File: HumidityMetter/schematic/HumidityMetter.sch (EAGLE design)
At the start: 65 parts, among them IC1 LM317, IC2 LM317, IC3 STM32F103C8T6, IC4 AM2320, J1 0, J2 0, J3 0, J4 0, K1 POWER_ON, T1 BSS84, T2 BC847, X1 +9V, X2 GND, X3 ISP

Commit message: Himidity metter. Board routed.
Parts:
- R24: device __MyCommonLib1:RSMD_0805 -> __MyCommonLib1:RSMD_1206_BIG_GAP
- R26, R27, R28, R29: device __MyCommonLib1:RSMD_0805 -> __MyCommonLib1:R0207
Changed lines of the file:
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@@
 <setting verticaltext="up"/>
 </settings>
-<grid distance="0.025" unitdist="inch" unit="inch" style="lines" multiple="4" display="yes" altdistance="0.01" altunitdist="inch" altunit="inch"/>
+<grid distance="0.1" unitdist="inch" unit="inch" style="lines" multiple="1" display="no" altdistance="0.01" altunitdist="inch" altunit="inch"/>
 <layers>
 <layer number="1" name="Top" color="4" fill="1" visible="yes" active="no"/>
@@
 <part name="R22" library="__MyCommonLib1" deviceset="R" device="SMD_0805" value="390R"/>
 <part name="R23" library="__MyCommonLib1" deviceset="R" device="SMD_0805" value="390R"/>
-<part name="R24" library="__MyCommonLib1" deviceset="R" device="SMD_0805" value="18K"/>
+<part name="R24" library="__MyCommonLib1" deviceset="R" device="SMD_1206_BIG_GAP" value="18K"/>
 <part name="R25" library="__MyCommonLib1" deviceset="R" device="SMD_0805" value="6K8"/>
 <part name="C9" library="__MyCommonLib1" deviceset="C" device="SMD_0805" value="0.1uF"/>
@@
 <part name="C1" library="__MyCommonLib1" deviceset="C" device="SMD_0805" value="0.1uF"/>
 <part name="GND28" library="supply1" deviceset="GND" device=""/>
-<part name="R26" library="__MyCommonLib1" deviceset="R" device="SMD_0805" value="4K7"/>
-<part name="R27" library="__MyCommonLib1" deviceset="R" device="SMD_0805" value="4K7"/>
-<part name="R28" library="__MyCommonLib1" deviceset="R" device="SMD_0805" value="200R"/>
-<part name="R29" library="__MyCommonLib1" deviceset="R" device="SMD_0805" value="200R"/>
+<part name="R26" library="__MyCommonLib1" deviceset="R" device="0207" value="4K7"/>
+<part name="R27" library="__MyCommonLib1" deviceset="R" device="0207" value="4K7"/>
+<part name="R28" library="__MyCommonLib1" deviceset="R" device="0207" value="200R"/>
+<part name="R29" library="__MyCommonLib1" deviceset="R" device="0207" value="200R"/>
 <part name="D10" library="__MyCommonLib1" deviceset="1N4001" device="DO-41_10MM" value="1N4007"/>
 <part name="GND29" library="supply1" deviceset="GND" device=""/>

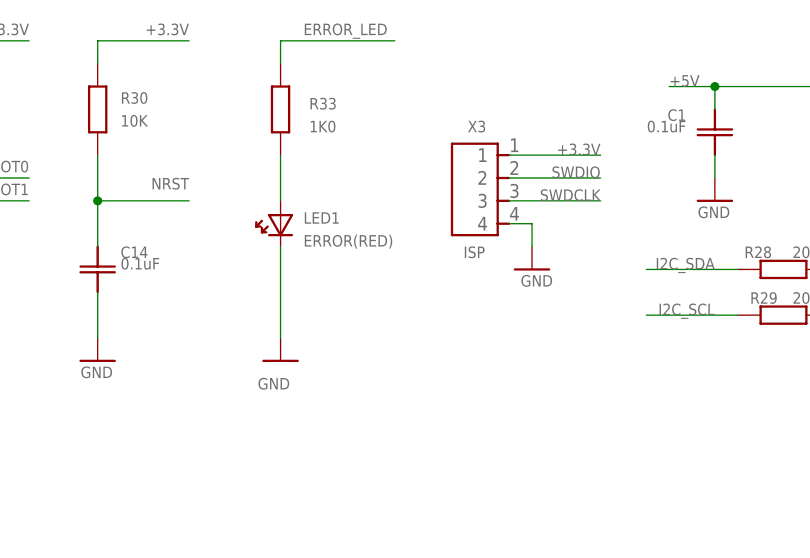
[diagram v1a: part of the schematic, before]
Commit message: Himidity metter. Board routed.
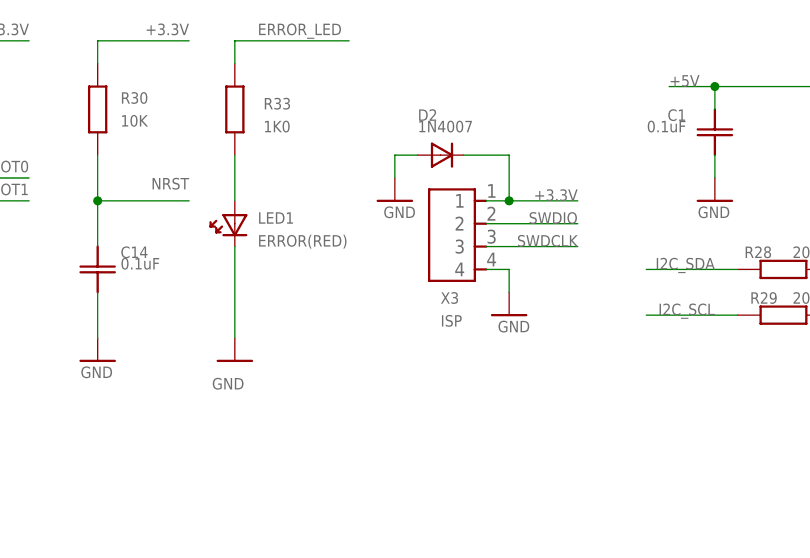
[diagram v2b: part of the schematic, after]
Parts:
- added D2: 1N4007, __MyCommonLib1:1N4001DO-41_10MM
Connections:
- net +3.3V: now also D2.CATHODE
- net GND: now also D2.ANODE
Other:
- moved on the sheet: LED1, R33, X3
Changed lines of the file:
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@@
 <setting verticaltext="up"/>
 </settings>
-<grid distance="0.1" unitdist="inch" unit="inch" style="lines" multiple="1" display="no" altdistance="0.01" altunitdist="inch" altunit="inch"/>
+<grid distance="0.1" unitdist="inch" unit="inch" style="lines" multiple="1" display="yes" altdistance="0.01" altunitdist="inch" altunit="inch"/>
 <layers>
 <layer number="1" name="Top" color="4" fill="1" visible="yes" active="no"/>
@@
 <part name="LED1" library="__MyCommonLib1" deviceset="LED3MM" device="(SMD0805)" value="ERROR(RED)"/>
 <part name="GND30" library="supply1" deviceset="GND" device=""/>
+<part name="D2" library="__MyCommonLib1" deviceset="1N4001" device="DO-41_10MM" value="1N4007"/>
+<part name="GND31" library="supply1" deviceset="GND" device=""/>
 </parts>
 <sheets>
@@
 <attribute name="VALUE" x="26.035" y="135.255" size="1.27" layer="96" font="vector" ratio="20"/>
 </instance>
-<instance part="X3" gate="G$1" x="68.58" y="157.48" smashed="yes" rot="MR0">
-<attribute name="NAME" x="71.12" y="162.56" size="1.27" layer="95" font="vector" ratio="20" rot="MR0"/>
-<attribute name="VALUE" x="68.58" y="149.86" size="1.27" layer="96" font="vector" ratio="20" rot="MR180"/>
-</instance>
-<instance part="GND26" gate="1" x="76.2" y="147.32" smashed="yes">
-<attribute name="VALUE" x="74.93" y="145.415" size="1.27" layer="96" font="vector" ratio="20"/>
+<instance part="X3" gate="G$1" x="66.04" y="152.4" smashed="yes" rot="MR0">
+<attribute name="NAME" x="66.04" y="144.78" size="1.27" layer="95" font="vector" ratio="20" rot="MR180"/>
+<attribute name="VALUE" x="66.04" y="142.24" size="1.27" layer="96" font="vector" ratio="20" rot="MR180"/>
+</instance>
+<instance part="GND26" gate="1" x="73.66" y="142.24" smashed="yes">
+<attribute name="VALUE" x="72.39" y="140.335" size="1.27" layer="96" font="vector" ratio="20"/>
 </instance>
 <instance part="IC4" gate="G$1" x="129.54" y="144.78" smashed="yes">
@@
 <attribute name="VALUE" x="170.18" y="162.56" size="1.27" layer="96" font="vector" ratio="20" rot="MR180"/>
 </instance>
-<instance part="R33" gate="R$1" x="48.26" y="165.1" smashed="yes" rot="R180">
-<attribute name="NAME" x="51.435" y="165.1" size="1.27" layer="95" font="vector" ratio="20"/>
-<attribute name="VALUE" x="51.435" y="162.56" size="1.27" layer="96" font="vector" ratio="20"/>
-</instance>
-<instance part="LED1" gate="LED$1" x="48.26" y="152.4" smashed="yes" rot="R180">
-<attribute name="NAME" x="50.8" y="152.4" size="1.27" layer="95" font="vector" ratio="20"/>
-<attribute name="VALUE" x="50.8" y="149.86" size="1.27" layer="96" font="vector" ratio="20"/>
-</instance>
-<instance part="GND30" gate="1" x="48.26" y="137.16" smashed="yes">
-<attribute name="VALUE" x="45.72" y="133.985" size="1.27" layer="96" font="vector" ratio="20"/>
+<instance part="R33" gate="R$1" x="43.18" y="165.1" smashed="yes" rot="R180">
+<attribute name="NAME" x="46.355" y="165.1" size="1.27" layer="95" font="vector" ratio="20"/>
+<attribute name="VALUE" x="46.355" y="162.56" size="1.27" layer="96" font="vector" ratio="20"/>
+</instance>
+<instance part="LED1" gate="LED$1" x="43.18" y="152.4" smashed="yes" rot="R180">
+<attribute name="NAME" x="45.72" y="152.4" size="1.27" layer="95" font="vector" ratio="20"/>
+<attribute name="VALUE" x="45.72" y="149.86" size="1.27" layer="96" font="vector" ratio="20"/>
+</instance>
+<instance part="GND30" gate="1" x="43.18" y="137.16" smashed="yes">
+<attribute name="VALUE" x="40.64" y="133.985" size="1.27" layer="96" font="vector" ratio="20"/>
+</instance>
+<instance part="D2" gate="D$1" x="66.04" y="160.02" smashed="yes" rot="R270">
+<attribute name="NAME" x="63.5" y="163.83" size="1.27" layer="95" font="vector" ratio="20"/>
+<attribute name="VALUE" x="63.5" y="162.56" size="1.27" layer="96" font="vector" ratio="20"/>
+</instance>
+<instance part="GND31" gate="1" x="60.96" y="154.94" smashed="yes">
+<attribute name="VALUE" x="59.69" y="153.035" size="1.27" layer="96" font="vector" ratio="20"/>
 </instance>
 </instances>
@@
 <pinref part="X3" gate="G$1" pin="4"/>
 <pinref part="GND26" gate="1" pin="GND"/>
-<wire x1="73.66" y1="152.4" x2="76.2" y2="152.4" width="0.1524" layer="91"/>
-<wire x1="76.2" y1="152.4" x2="76.2" y2="149.86" width="0.1524" layer="91"/>
+<wire x1="71.12" y1="147.32" x2="73.66" y2="147.32" width="0.1524" layer="91"/>
+<wire x1="73.66" y1="147.32" x2="73.66" y2="144.78" width="0.1524" layer="91"/>
 </segment>
 <segment>
@@
 <pinref part="LED1" gate="LED$1" pin="CATHODE"/>
 <pinref part="GND30" gate="1" pin="GND"/>
-<wire x1="48.26" y1="139.7" x2="48.26" y2="149.86" width="0.1524" layer="91"/>
+<wire x1="43.18" y1="139.7" x2="43.18" y2="149.86" width="0.1524" layer="91"/>
+</segment>
+<segment>
+<pinref part="D2" gate="D$1" pin="ANODE"/>
+<pinref part="GND31" gate="1" pin="GND"/>
+<wire x1="63.5" y1="160.02" x2="60.96" y2="160.02" width="0.1524" layer="91"/>
+<wire x1="60.96" y1="160.02" x2="60.96" y2="157.48" width="0.1524" layer="91"/>
 </segment>
 </net>
@@
 <segment>
 <pinref part="X3" gate="G$1" pin="1"/>
-<wire x1="83.82" y1="160.02" x2="73.66" y2="160.02" width="0.1524" layer="91"/>
-<label x="83.82" y="161.29" size="1.27" layer="95" font="vector" ratio="20" rot="R180"/>
+<wire x1="81.28" y1="154.94" x2="73.66" y2="154.94" width="0.1524" layer="91"/>
+<label x="81.28" y="156.21" size="1.27" layer="95" font="vector" ratio="20" rot="R180"/>
+<pinref part="D2" gate="D$1" pin="CATHODE"/>
+<wire x1="73.66" y1="154.94" x2="71.12" y2="154.94" width="0.1524" layer="91"/>
+<wire x1="68.58" y1="160.02" x2="73.66" y2="160.02" width="0.1524" layer="91"/>
+<wire x1="73.66" y1="160.02" x2="73.66" y2="154.94" width="0.1524" layer="91"/>
+<junction x="73.66" y="154.94"/>
 </segment>
 <segment>
@@
 <segment>
 <pinref part="X3" gate="G$1" pin="2"/>
-<wire x1="83.82" y1="157.48" x2="73.66" y2="157.48" width="0.1524" layer="91"/>
-<label x="83.82" y="158.75" size="1.27" layer="95" font="vector" ratio="20" rot="R180"/>
+<wire x1="81.28" y1="152.4" x2="71.12" y2="152.4" width="0.1524" layer="91"/>
+<label x="81.28" y="153.67" size="1.27" layer="95" font="vector" ratio="20" rot="R180"/>
 </segment>
 <segment>
@@
 <segment>
 <pinref part="X3" gate="G$1" pin="3"/>
-<wire x1="83.82" y1="154.94" x2="73.66" y2="154.94" width="0.1524" layer="91"/>
-<label x="83.82" y="156.21" size="1.27" layer="95" font="vector" ratio="20" rot="R180"/>
+<wire x1="81.28" y1="149.86" x2="71.12" y2="149.86" width="0.1524" layer="91"/>
+<label x="81.28" y="151.13" size="1.27" layer="95" font="vector" ratio="20" rot="R180"/>
 </segment>
 <segment>
@@
 <segment>
 <pinref part="R33" gate="R$1" pin="PIN0"/>
-<wire x1="48.26" y1="170.18" x2="48.26" y2="172.72" width="0.1524" layer="91"/>
-<wire x1="48.26" y1="172.72" x2="60.96" y2="172.72" width="0.1524" layer="91"/>
-<label x="50.8" y="173.355" size="1.27" layer="95" font="vector" ratio="20"/>
+<wire x1="43.18" y1="170.18" x2="43.18" y2="172.72" width="0.1524" layer="91"/>
+<wire x1="43.18" y1="172.72" x2="55.88" y2="172.72" width="0.1524" layer="91"/>
+<label x="45.72" y="173.355" size="1.27" layer="95" font="vector" ratio="20"/>
 </segment>
 </net>
@@
 <pinref part="R33" gate="R$1" pin="PIN1"/>
 <pinref part="LED1" gate="LED$1" pin="ANODE"/>
-<wire x1="48.26" y1="160.02" x2="48.26" y2="154.94" width="0.1524" layer="91"/>
-</segment>
-</net>
+<wire x1="43.18" y1="160.02" x2="43.18" y2="154.94" width="0.1524" layer="91"/>
+</segment>
+</net>

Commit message: Himidity metter. Board routed. Fix tiny problems.
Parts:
- LCD1: device __MyCommonLib1:LCD_0802B(0802B) -> __MyCommonLib1:LCD_0802B(0802B_CHINA_CLONE)
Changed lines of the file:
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@@
 <setting verticaltext="up"/>
 </settings>
-<grid distance="0.1" unitdist="inch" unit="inch" style="lines" multiple="1" display="yes" altdistance="0.01" altunitdist="inch" altunit="inch"/>
+<grid distance="0.1" unitdist="inch" unit="inch" style="lines" multiple="1" display="no" altdistance="0.01" altunitdist="inch" altunit="inch"/>
 <layers>
 <layer number="1" name="Top" color="4" fill="1" visible="yes" active="no"/>
@@
 <part name="FRAME1" library="frames" deviceset="A4L-LOC" device="" value="HUMIDITY METTER"/>
 <part name="IC3" library="__MyCommonLib1" deviceset="STM32F103C8T6(LQFP48)" device="(LQFP48)" value="STM32F103C8T6"/>
-<part name="LCD1" library="__MyCommonLib1" deviceset="LCD_0802B" device="(0802B)" value="LCD_0802B"/>
+<part name="LCD1" library="__MyCommonLib1" deviceset="LCD_0802B" device="(0802B_CHINA_CLONE)" value="LCD_0802B"/>
 <part name="IC1" library="__MyCommonLib1" deviceset="LM317" device="(D2PAK)" value="LM317"/>
 <part name="X1" library="__MyCommonLib1" deviceset="PIN1X1" device="3.5MM_DRILL" value="+9V"/>
